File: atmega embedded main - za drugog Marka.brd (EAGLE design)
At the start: 311.1 x 125.9 mm, 152 parts, among them IC1 ATMEGA328PROUND, K1 SWITCH, K100 SWITCH, K101 SWITCH, K102 SWITCH, K103 SWITCH, K104 SWITCH, K105 SWITCH, K106 SWITCH, K107 SWITCH, K108 SWITCH, K109 SWITCH, K110 SWITCH, K111 SWITCH, K112 SWITCH, K113 SWITCH, K114 SWITCH, K115 SWITCH, K116 SWITCH, K117 SWITCH, K118 SWITCH, K119 SWITCH, K120 SWITCH, K121 SWITCH, K122 SWITCH, K123 SWITCH, K124 SWITCH, K125 SWITCH, K126 SWITCH, K127 SWITCH, K128 SWITCH, K2 SWITCH, K3 SWITCH, K60 SWITCH, K67 SWITCH, K68 SWITCH, K69 SWITCH, K70 SWITCH, K71 SWITCH, K72 SWITCH, K73 SWITCH, K74 SWITCH, K75 SWITCH, K76 SWITCH, K77 SWITCH, K78 SWITCH, K79 SWITCH, K80 SWITCH, K81 SWITCH, K82 SWITCH, K83 SWITCH, K84 SWITCH, K85 SWITCH, K86 SWITCH, K87 SWITCH, K88 SWITCH, K89 SWITCH, K90 SWITCH, K91 SWITCH, K92 SWITCH, K93 SWITCH, K94 SWITCH, K95 SWITCH, K96 SWITCH, K97 SWITCH, K98 SWITCH, K99 SWITCH

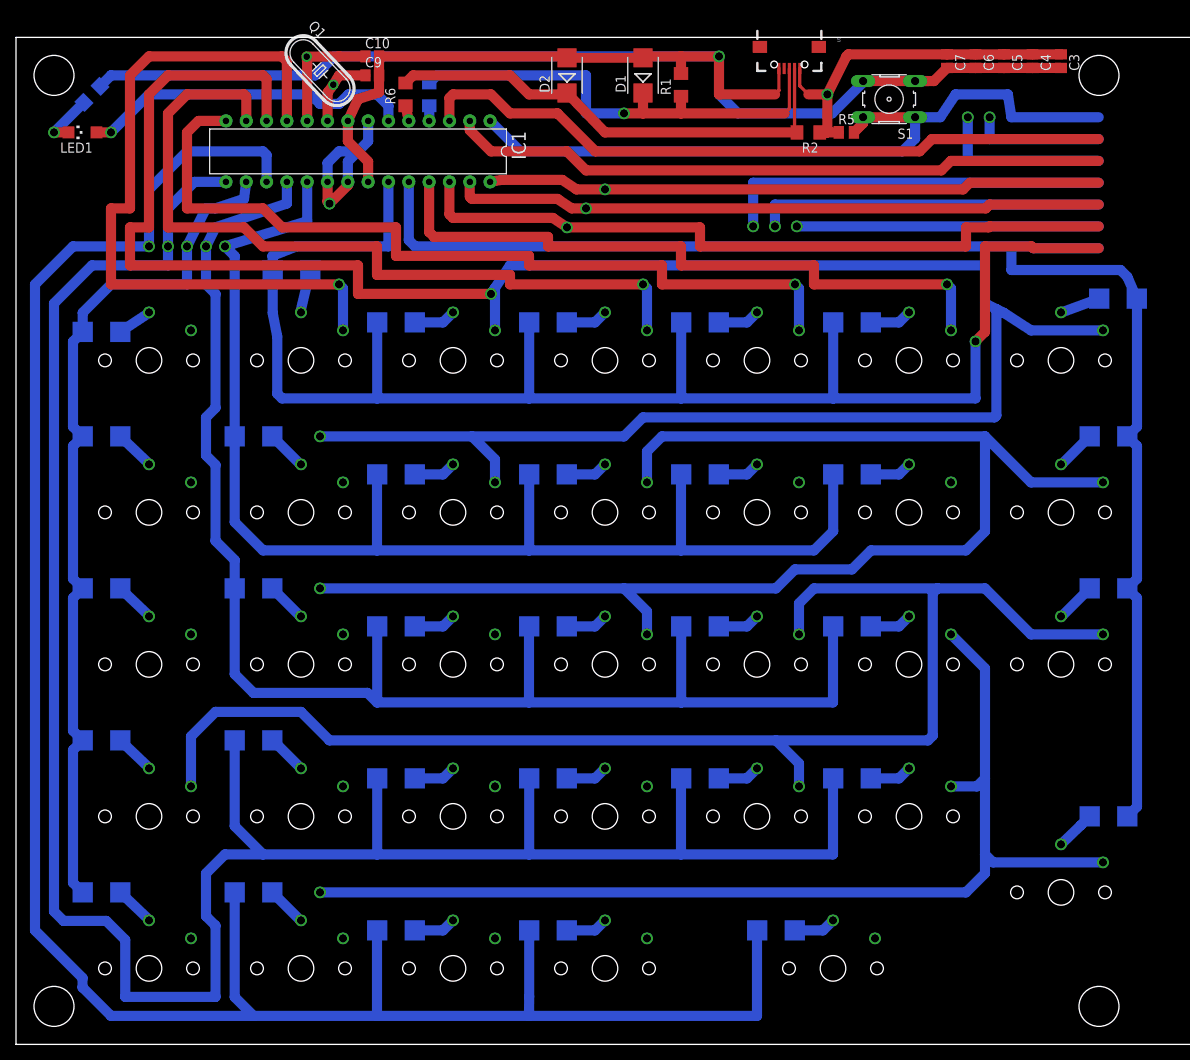
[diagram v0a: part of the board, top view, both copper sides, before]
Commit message: Test 1
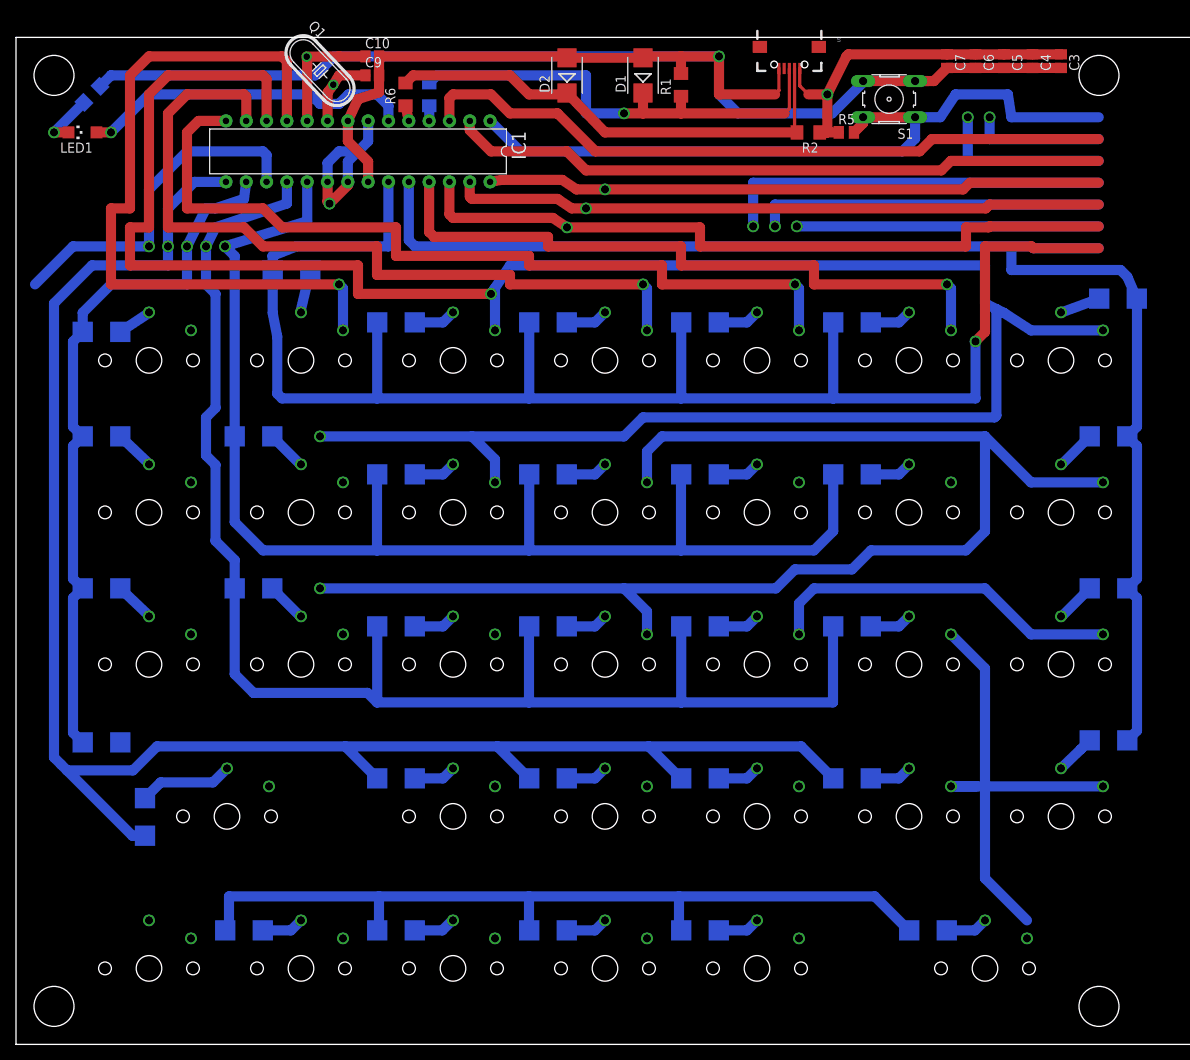
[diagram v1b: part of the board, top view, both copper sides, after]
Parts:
- moved D87 23.8 mm to (21.4, 4.75)
- moved D84 19.0 mm to (59.4, 4.75)
- moved D85 19.0 mm to (78.4, 4.75)
- moved D86 19.0 mm to (106.9, 4.75)
- moved K88 19.0 mm to (28.5, 0.00)
- moved K94 19.0 mm to (47.5, 0.00)
- moved K95 19.0 mm to (66.5, 0.00)
- moved K96 19.0 mm to (85.5, 0.00)
- moved K97 19.0 mm to (114.0, 0.00)
- moved D82 18.8 mm to (3.56, 28.2)
- moved D83 18.4 mm to (40.4, 4.75)
- moved D81 11.0 mm to (9.00, 18.9), turned to 270 degrees
- moved K87 9.75 mm to (19.2, 19.0)
- moved D97 9.50 mm to (129.4, 28.5)
- moved K92 9.50 mm to (123.5, 19.0)
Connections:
- net COL1: now also K87.P$2; no longer K94.P$2
- net COL2: now also K94.P$2; no longer K95.P$2
- net COL3: now also K95.P$2; no longer K96.P$2
- net COL4: now also K96.P$2; no longer K87.P$2, K97.P$2
- net ROW4: now also D81.A; no longer D87.A
- net ROW5: now also D87.A; no longer D86.A
- net ROW6: no longer D81.A
- net ROW7: now also D86.A
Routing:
- net COL4: track 365.8 -> 191.6 mm
- net ROW5: track 779.7 -> 659.4 mm
- net COL5: track 276.8 -> 185.9 mm, vias 2 -> 1
- net ROW4: track 803.6 -> 737.7 mm
- net COL1: track 191.8 -> 152.7 mm
- net COL3: track 371.8 -> 351.9 mm
- net ROW6: track 447.1 -> 427.3 mm
- net COL2: track 387.8 -> 368.3 mm
- net ROW7: track 276.3 -> 266.8 mm
- net N$4: track 5.16 -> 11.8 mm
- net N$5: track 5.16 -> 0.18 mm
